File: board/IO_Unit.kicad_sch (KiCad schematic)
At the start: 2 parts, among them U3 MCP23017_SS, U5 TCA9548APWR

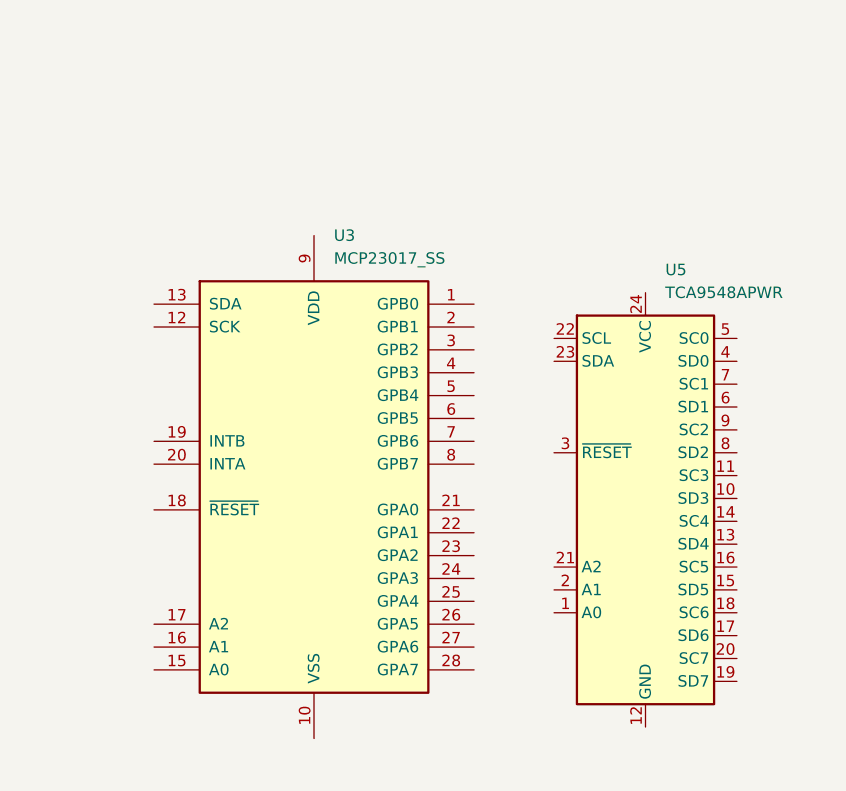
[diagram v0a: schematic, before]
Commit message: [6-5-2024] Create I/O
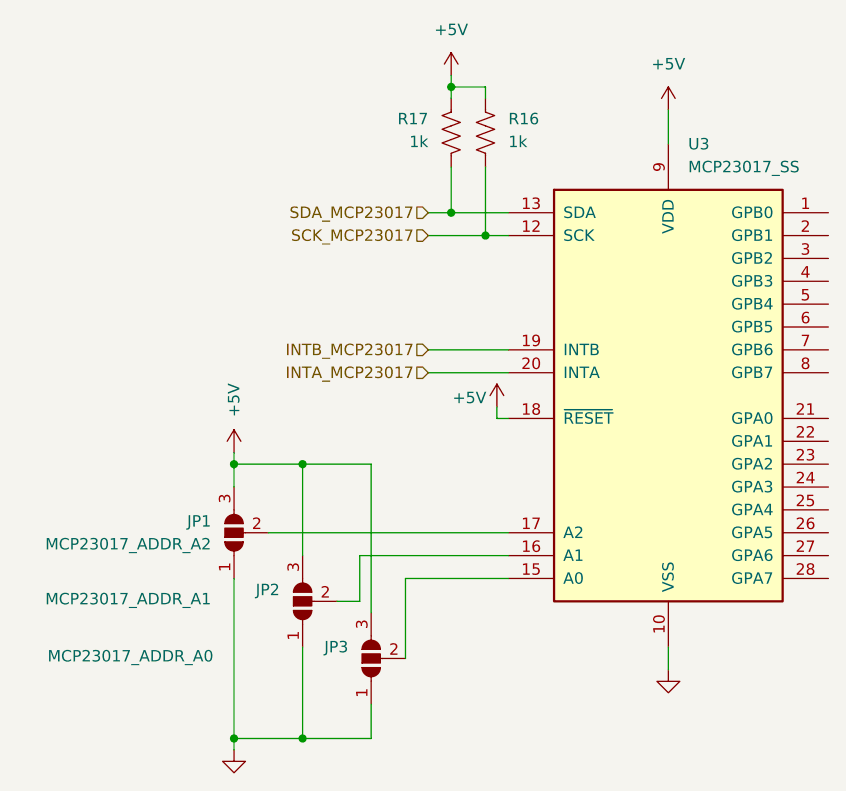
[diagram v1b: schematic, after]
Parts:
- removed U5: TCA9548APWR, Package_SO:TSSOP-24_4.4x7.8mm_P0.65mm, symbol Interface_Expansion:TCA9548APWR
- added JP1: MCP23017_ADDR_A2, Jumper:SolderJumper-3_P1.3mm_Open_Pad1.0x1.5mm_NumberLabels, symbol Jumper:SolderJumper_3_Open
- added JP2: MCP23017_ADDR_A1, Jumper:SolderJumper-3_P1.3mm_Open_Pad1.0x1.5mm_NumberLabels, symbol Jumper:SolderJumper_3_Open
- added JP3: MCP23017_ADDR_A0, Jumper:SolderJumper-3_P1.3mm_Open_Pad1.0x1.5mm_NumberLabels, symbol Jumper:SolderJumper_3_Open
- added R16, R17: 1k, Resistor_SMD:R_0805_2012Metric_Pad1.20x1.40mm_HandSolder, symbol Device:R_US
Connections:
- net GND: now reaches U3.10 (VSS)
- net GND: now also JP1.1 (A), JP2.1 (A), JP3.1 (A)
- net SCK_MCP23017: now reaches U3.12 (SCK)
- net SCK_MCP23017: now also R16.2
- net SDA_MCP23017: now reaches U3.13 (SDA)
- net SDA_MCP23017: now also R17.2
- net at U3.15 (A0): now also JP3.2 (C)
- net at U3.16 (A1): now also JP2.2 (C)
- net at U3.17 (A2): now also JP1.2 (C)
- net +5V: now reaches U3.18 (~{RESET})
- net +5V: now also U3.9 (VDD), JP1.3 (B), JP2.3 (B), JP3.3 (B), R16.1, R17.1
- net INTB_MCP23017: now reaches U3.19 (INTB)
- net INTA_MCP23017: now reaches U3.20 (INTA)
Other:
- moved on the sheet: U3
